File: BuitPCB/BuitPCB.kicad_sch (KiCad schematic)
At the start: 0 parts

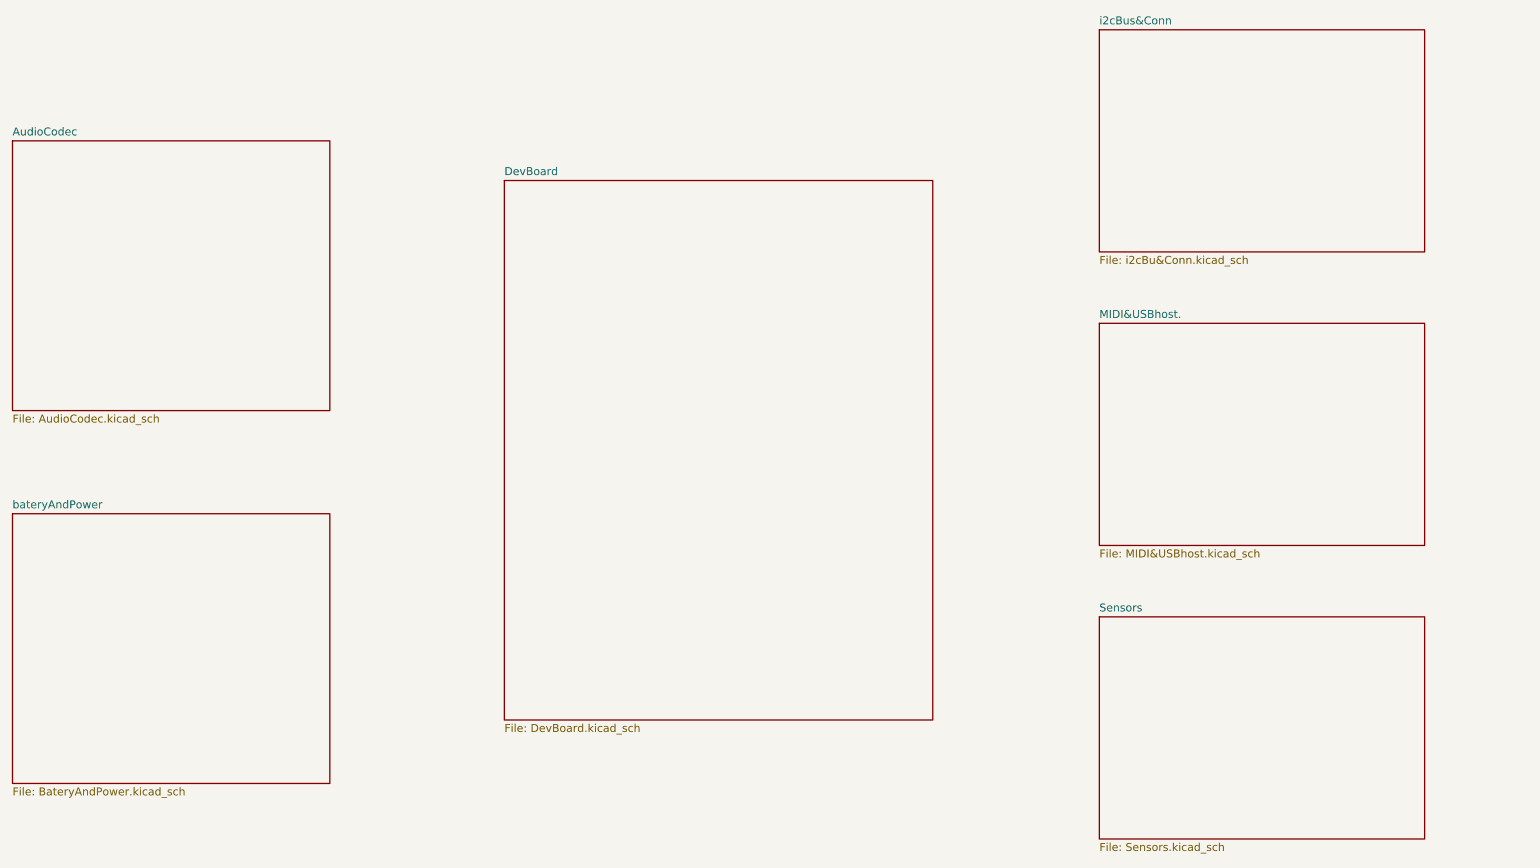
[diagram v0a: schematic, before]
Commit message: Updated almost to final 0.1 version
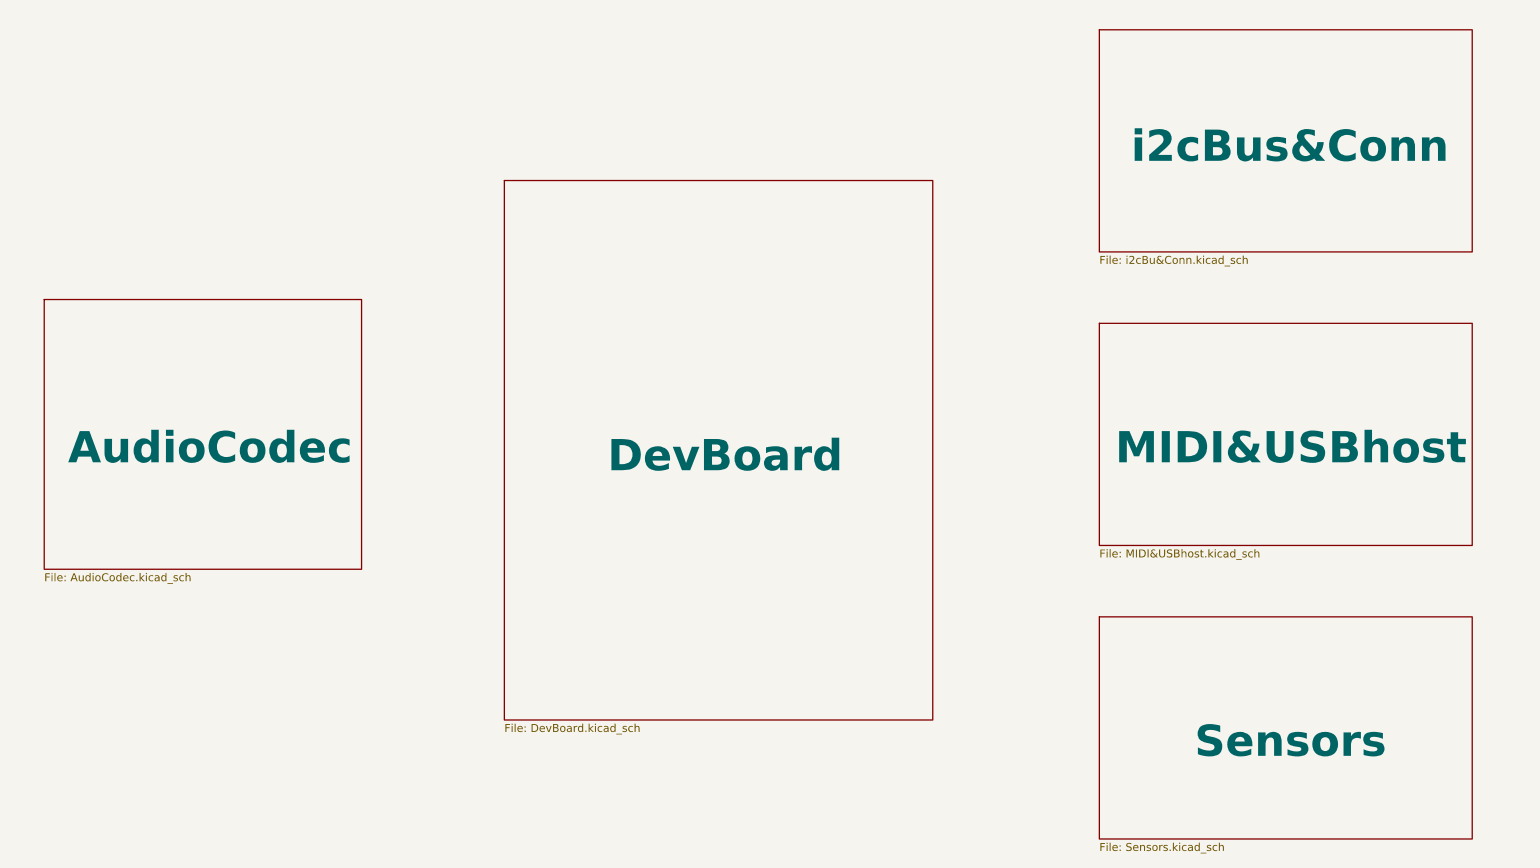
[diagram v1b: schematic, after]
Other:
- sheet MIDI&USBhost. renamed MIDI&USBhost
- removed sheet bateryAndPower

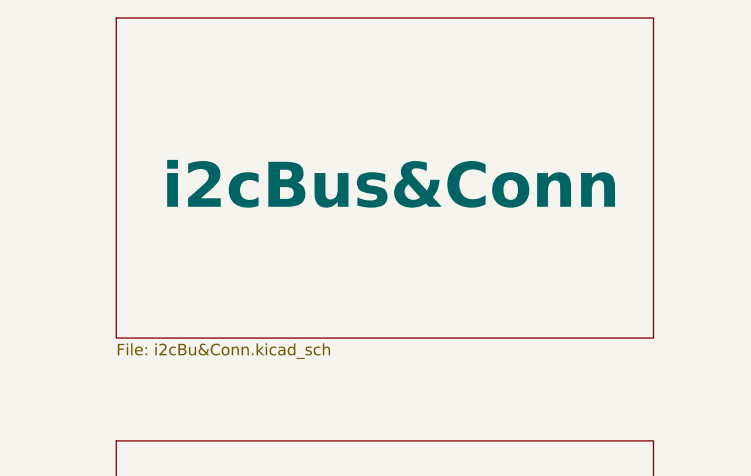
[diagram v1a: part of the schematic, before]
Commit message: Updated and send to fab
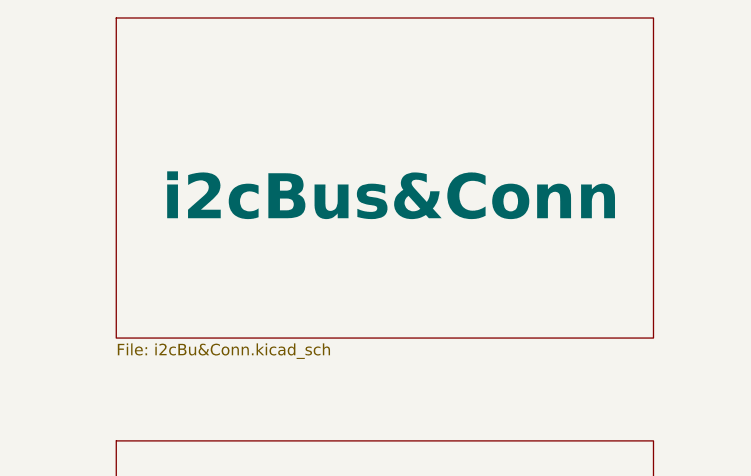
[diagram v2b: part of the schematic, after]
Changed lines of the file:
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@@
     (stroke (width 0) (type solid) (color 0 0 0 0))
     (fill (color 0 0 0 0.0000))
-    (property "Sheet name" "i2cBus&Conn" (id 0) (at 212.09 45.72 0)
+    (property "Sheet name" "i2cBus&Conn" (id 0) (at 212.09 46.99 0)
       (effects (font (size 5 5) bold) (justify left bottom))
     )
